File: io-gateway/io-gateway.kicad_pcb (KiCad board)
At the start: 4 copper layers, 155 x 81.5 mm, 90 parts, among them J1 1752201, J2 1752201, J3 1752201, J4 Screw_Terminal_01x09, J5 Screw_Terminal_01x09, J6 Screw_Terminal_01x09, K1 2071556-2, K2 2071556-2, K3 2071556-2, K4 2071556-2, K5 2071556-2, K6 2071556-2, K7 2071556-2, K8 2071556-2, K9 2071556-2, U3 TPS54308

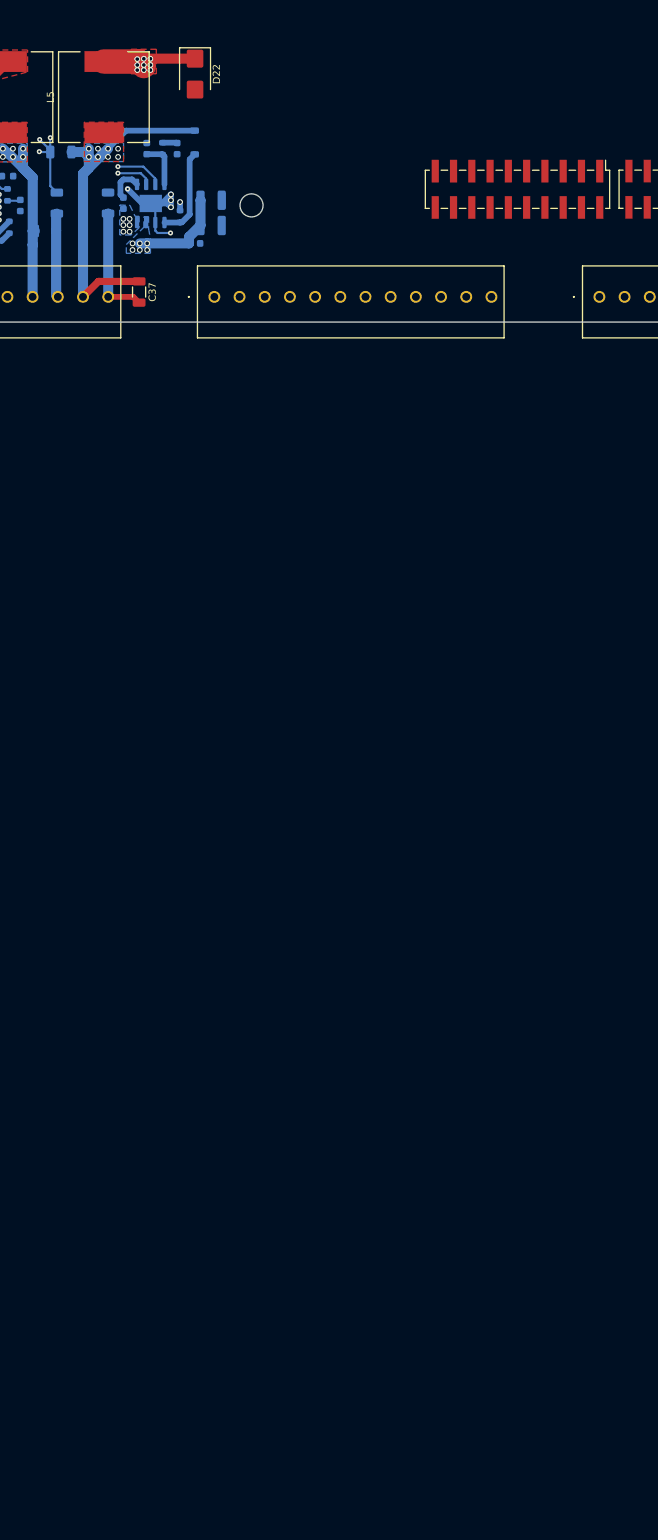
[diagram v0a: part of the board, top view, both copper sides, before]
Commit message: temp
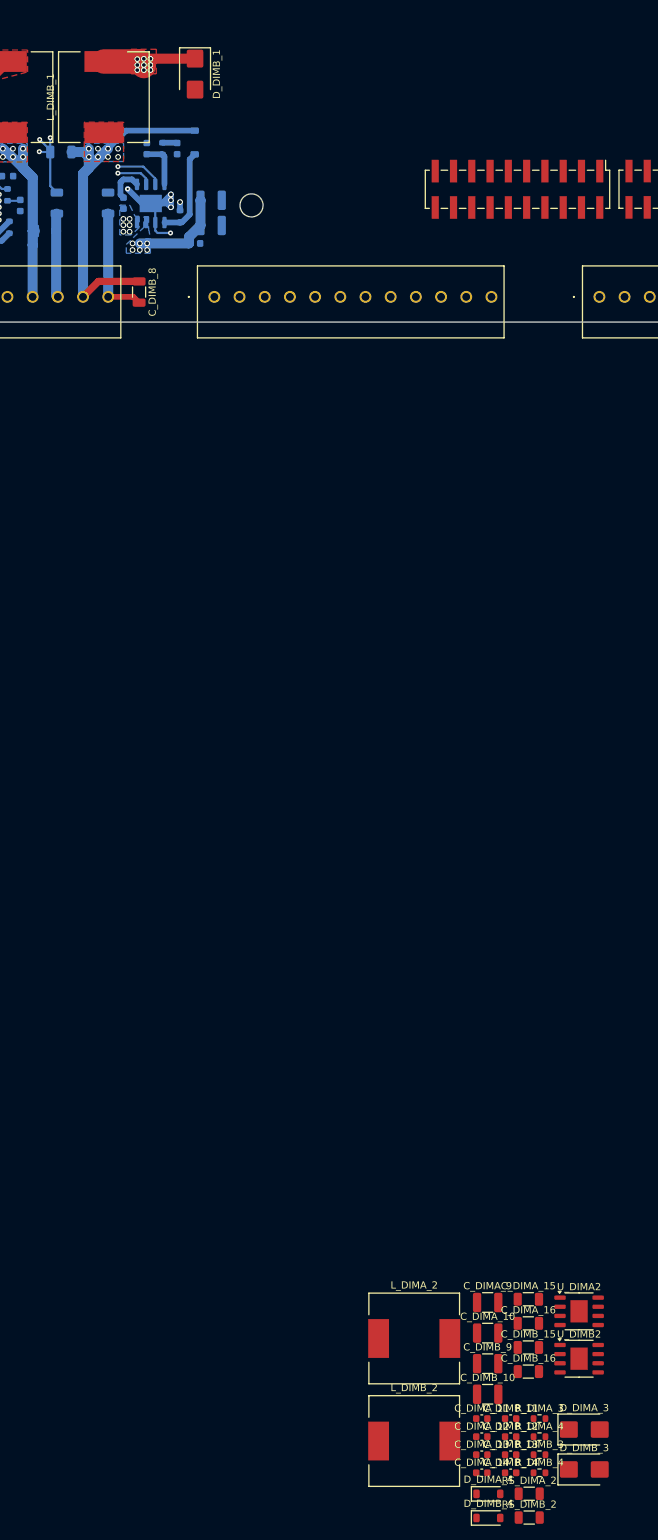
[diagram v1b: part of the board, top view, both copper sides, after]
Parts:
- added C_DIMA_10: 10µF 50V, Capacitor_SMD:C_1210_3225Metric, F.Cu at (146.5, 270.2)
- added C_DIMA_11: 470pF, Capacitor_SMD:C_0603_1608Metric, F.Cu at (145.7, 282.1)
- added C_DIMA_12: 100nF 50V, Capacitor_SMD:C_0603_1608Metric, F.Cu at (145.7, 284.6)
- added C_DIMA_13: 22pF, Capacitor_SMD:C_0603_1608Metric, F.Cu at (145.7, 287.1)
- added C_DIMA_14: 100nF 50V, Capacitor_SMD:C_0603_1608Metric, F.Cu at (145.7, 289.6)
- added C_DIMA_15: 1µF 50V, Capacitor_SMD:C_1206_3216Metric, F.Cu at (152.1, 265.5)
- added C_DIMA_16: NM, Capacitor_SMD:C_1206_3216Metric, F.Cu at (152.1, 268.9)
- added C_DIMA_9: 10µF 50V, Capacitor_SMD:C_1210_3225Metric, F.Cu at (146.5, 266.0)
- added C_DIMB_10: 10µF 50V, Capacitor_SMD:C_1210_3225Metric, F.Cu at (146.5, 278.7)
- added C_DIMB_11: 470pF, Capacitor_SMD:C_0603_1608Metric, F.Cu at (149.7, 282.1)
- added C_DIMB_12: 100nF 50V, Capacitor_SMD:C_0603_1608Metric, F.Cu at (149.7, 284.6)
- added C_DIMB_13: 22pF, Capacitor_SMD:C_0603_1608Metric, F.Cu at (149.7, 287.1)
- added C_DIMB_14: 100nF 50V, Capacitor_SMD:C_0603_1608Metric, F.Cu at (149.7, 289.6)
- added C_DIMB_15: 1µF 50V, Capacitor_SMD:C_1206_3216Metric, F.Cu at (152.1, 272.2)
- added C_DIMB_16: NM, Capacitor_SMD:C_1206_3216Metric, F.Cu at (152.1, 275.6)
- added C_DIMB_9: 10µF 50V, Capacitor_SMD:C_1210_3225Metric, F.Cu at (146.5, 274.5)
- added D_DIMA_3: D_Schottky, Diode_SMD:D_SMB, F.Cu at (159.9, 283.6)
- added D_DIMA_4: D_Zener, Diode_SMD:D_SOD-123, F.Cu at (146.6, 292.6)
- added D_DIMB_3: D_Schottky, Diode_SMD:D_SMB, F.Cu at (159.9, 289.2)
- added D_DIMB_4: D_Zener, Diode_SMD:D_SOD-123, F.Cu at (146.6, 295.9)
- added L_DIMA_2: 47µH 3.8A, Inductor_SMD:L_12x12mm_H8mm, F.Cu at (136.3, 271.0)
- added L_DIMB_2: 47µH 3.8A, Inductor_SMD:L_12x12mm_H8mm, F.Cu at (136.3, 285.2)
- added RS_DIMA_2: R, Resistor_SMD:R_1206_3216Metric, F.Cu at (152.2, 292.5)
- added RS_DIMB_2: R, Resistor_SMD:R_1206_3216Metric, F.Cu at (152.2, 295.9)
- added R_DIMA_3: 24k9, Resistor_SMD:R_0603_1608Metric, F.Cu at (153.7, 282.1)
- added R_DIMA_4: 47k, Resistor_SMD:R_0603_1608Metric, F.Cu at (153.7, 284.6)
- added R_DIMB_3: 24k9, Resistor_SMD:R_0603_1608Metric, F.Cu at (153.7, 287.1)
- added R_DIMB_4: 47k, Resistor_SMD:R_0603_1608Metric, F.Cu at (153.7, 289.6)
- added U_DIMA2: LED5000, Package_SO:HSOP-8-1EP_3.9x4.9mm_P1.27mm_EP2.41x3.1mm, F.Cu at (159.2, 267.2)
- added U_DIMB2: LED5000, Package_SO:HSOP-8-1EP_3.9x4.9mm_P1.27mm_EP2.41x3.1mm, F.Cu at (159.2, 273.8)
- renumbered C30 to C_DIMB_1, C31 to C_DIMB_2, C33 to C_DIMB_3, C32 to C_DIMB_4, C34 to C_DIMB_5, C35 to C_DIMB_6, C36 to C_DIMB_7, C37 to C_DIMB_8, D22 to D_DIMB_1, D23 to D_DIMB_2, L5 to L_DIMB_1, RS_DIM2 to RS_DIMB_1, R40 to R_DIMB_1, R41 to R_DIMB_2
